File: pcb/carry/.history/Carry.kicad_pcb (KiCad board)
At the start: 2 copper layers, 22.9 x 30.5 mm, 9 parts, among them J2 Conn_01x02, U1 Luckfox-Pico_Mini_B, U2 MCP73831-2-OT

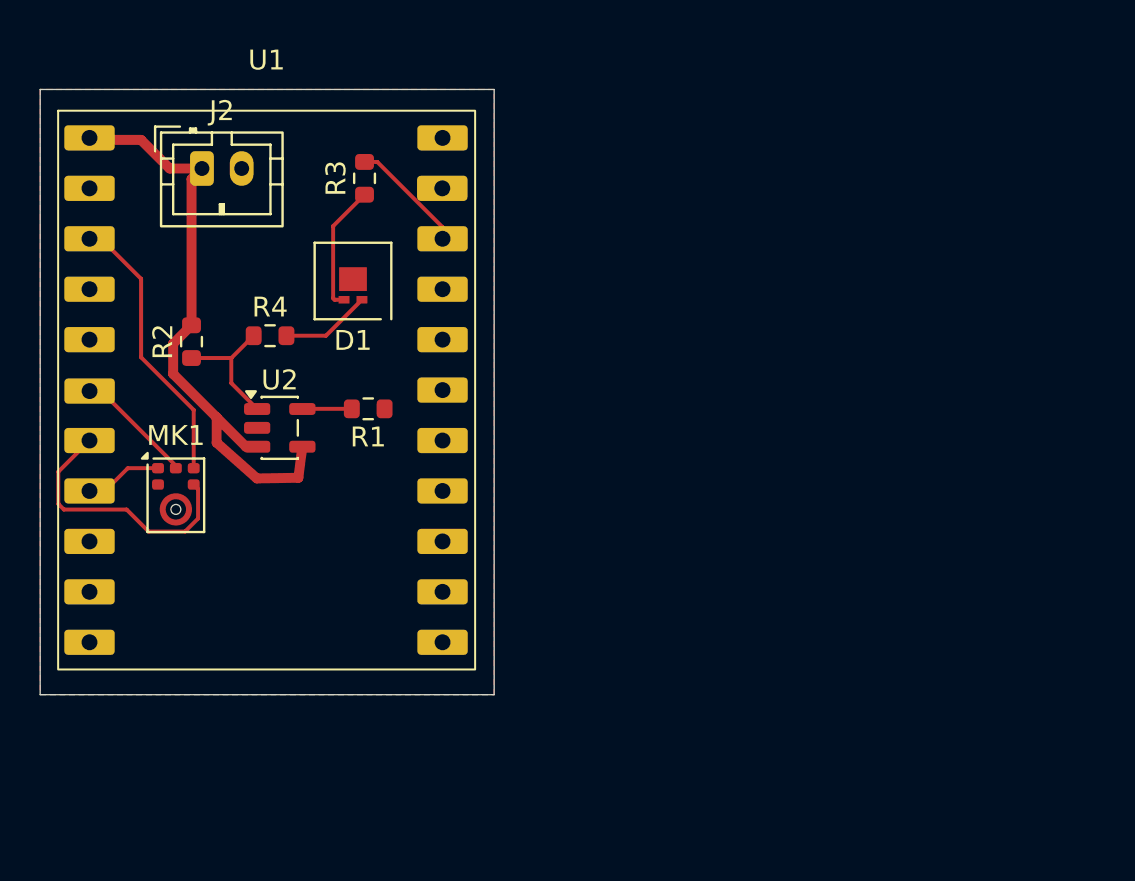
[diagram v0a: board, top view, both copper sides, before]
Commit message: updated
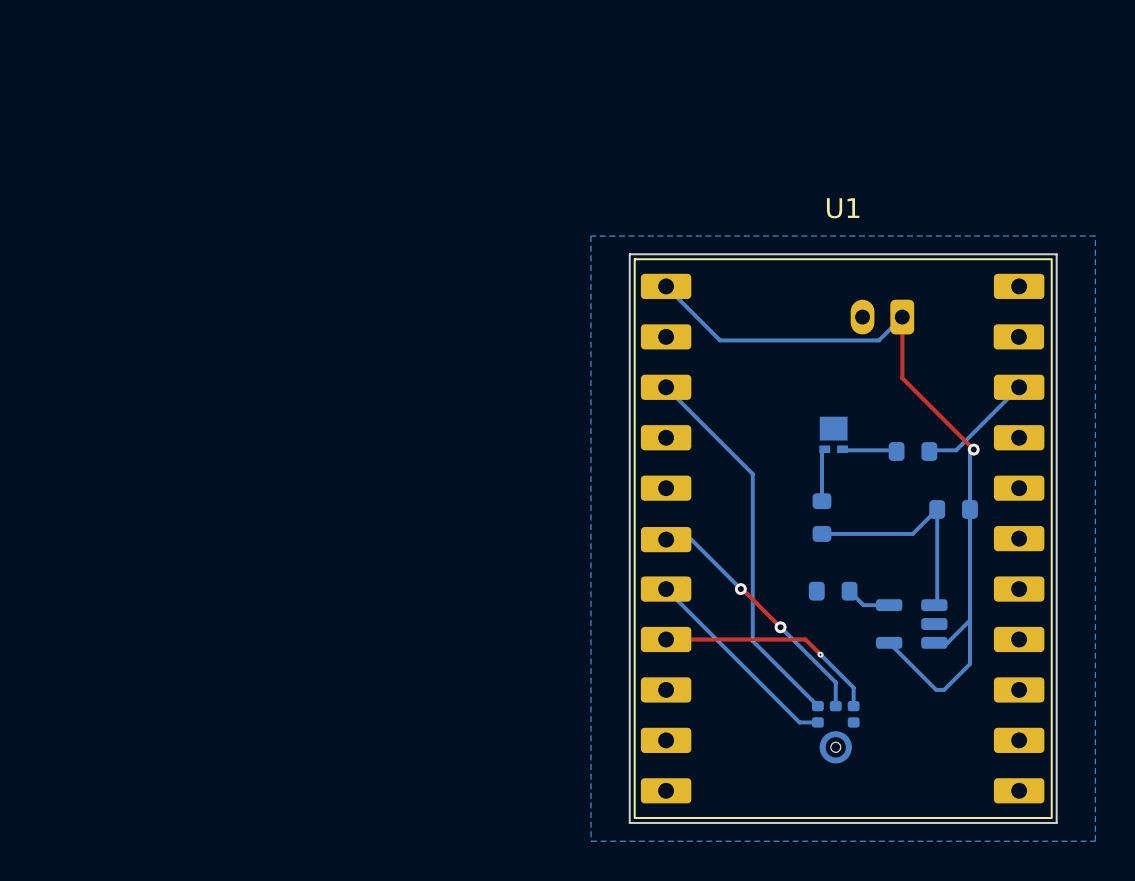
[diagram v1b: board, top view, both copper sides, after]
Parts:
- D1, J2, MK1, R1, R2, R3, R4, U2: moved to B.Cu
- moved R2 39.3 mm to (145.1, 89.7), turned to 0 degrees
- moved J2 36.1 mm to (142.5, 80.0), turned to 180 degrees
- moved MK1 35.3 mm to (139.1, 101.0), turned to 180 degrees
- moved U2 33.3 mm to (143.0, 95.5), turned to 180 degrees
- moved R3 30.9 mm to (143.0, 86.8), turned to 0 degrees
- moved U1 30.0 mm to (139.5, 91.2)
- moved R4 29.3 mm to (138.4, 90.1), turned to 90 degrees
- moved D1 25.4 mm to (139.0, 86.2), turned to 180 degrees
- moved R1 25.2 mm to (139.0, 93.8), turned to 0 degrees
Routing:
- net Net-(J1-Pin_1): track 31.0 -> 40.5 mm, vias 0 -> 1
- net Net-(MK1-WS): track 3.92 -> 11.4 mm, vias 0 -> 1
- net /MIC_DATA: track 6.02 -> 13.3 mm, vias 0 -> 2
- net Net-(MK1-VDD): track 14.1 -> 19.8 mm
- net Net-(U2-STAT): track 6.70 -> 11.2 mm
- net Net-(D1-A2): track 6.45 -> 2.77 mm
- net Net-(MK1-BCLK): track 13.5 -> 10.4 mm
- net Net-(D1-A1): track 4.55 -> 2.67 mm
- added copper zone on B.Cu, net GND
- removed copper zone on F.Cu, net Net-(MK1-BCLK)
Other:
- board size 22.9 x 30.5 mm -> 21.5 x 28.6 mm
